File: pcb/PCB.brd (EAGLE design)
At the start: 42.5 x 42.5 mm, 18 parts

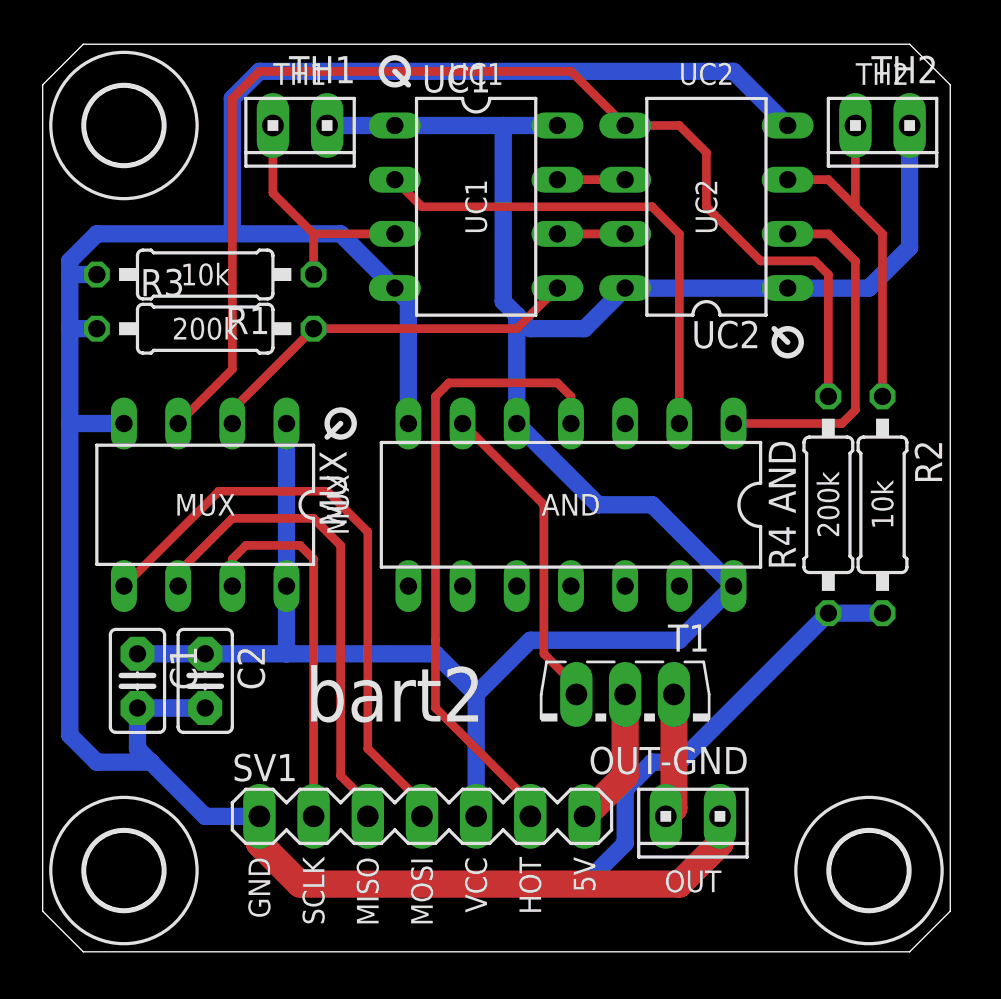
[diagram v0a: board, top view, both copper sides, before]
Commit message: Updated pcb
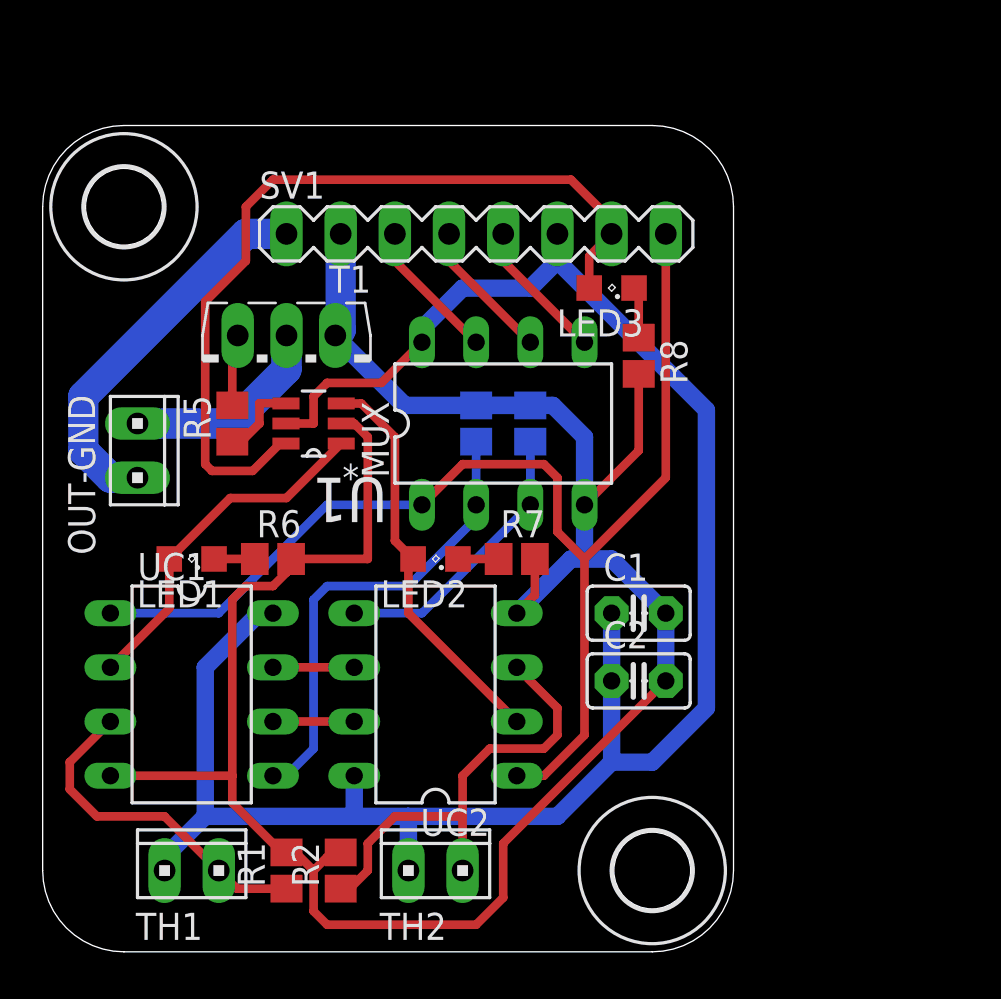
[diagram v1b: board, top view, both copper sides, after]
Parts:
- removed AND: 74HC21N, 74xx-eu:DIL14
- removed H2: MOUNT-HOLE3.6, holes:3,6
- added LED1, LED2, LED3: (no value), led:SML0805
- added R5: 1k, resistor:R0805
- added R6, R7, R8: 100, resistor:R0805
- added U1: SN74LVC1G11DBVR, parts:SOT95P280X145-6N
- R1, R2: device resistor:0207/10 -> resistor:R0805
- R3, R4: value 200k -> 100k; device resistor:0207/10 -> resistor:R0805
- SV1: device parts:MA07-1 -> parts:MA08-1
- moved TH2 40.7 mm to (18.4, 3.81), turned to 0 degrees
- moved TH1 35.3 mm to (6.99, 3.81), turned to 0 degrees
- moved OUT-GND 31.2 mm to (4.45, 23.5), turned to 270 degrees
- moved R2 30.6 mm to (14.0, 3.81), turned to 90 degrees
- moved R1 28.2 mm to (11.4, 3.81), turned to 90 degrees
- moved SV1 27.4 mm to (20.3, 33.7)
- moved UC1 26.5 mm to (6.99, 12.1)
- moved UC2 26.2 mm to (18.4, 12.1)
- moved C1 23.7 mm to (27.9, 15.9), turned to 0 degrees
- moved T1 23.1 mm to (11.4, 27.6)
- moved C2 20.3 mm to (27.9, 12.7), turned to 0 degrees
- moved MUX 14.5 mm to (21.6, 24.8), turned to 0 degrees
- moved R4 14.5 mm to (22.9, 24.8), flipped to the bottom, turned to 270 degrees
- moved R3 13.5 mm to (20.3, 24.8), flipped to the bottom, turned to 270 degrees
- moved H1 10.2 mm to (28.6, 3.81)
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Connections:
- new net N$2: LED3.C, R8.1
- new net N$3: R5.1, U1.4
- new net N$5: LED2.C, R7.1
- new net N$6: LED1.C, R6.1
- new net NRST: MUX.1, SV1.8, UC1.1, UC2.1
- net 5V: now also OUT-GND.1, SV1.1; no longer SV1.7, T1.2
- net GND: now also R6.2, R7.2, R8.2, SV1.2, T1.1, U1.2; no longer AND.7, OUT-GND.2, SV1.1
- net HOT: now also LED3.A, SV1.7, U1.6; no longer AND.4, SV1.6
- net MISO: now also SV1.4; no longer SV1.3
- net MOSI: now also SV1.5; no longer SV1.4
- net N$1: now also OUT-GND.2, T1.2; no longer OUT-GND.1, T1.1
- net N$4: now also R5.2; no longer AND.6
- net OUT1: now also LED1.A, U1.1; no longer AND.2
- net OUT2: now also LED2.A, U1.3; no longer AND.1
- net SCLK: now also SV1.3; no longer SV1.2
- net VCC: now also SV1.6, U1.5; no longer AND.14, AND.5, MUX.1, SV1.5, UC1.1, UC2.1
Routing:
- net NRST: track 0.00 -> 57.5 mm
- net GND: track 164.9 -> 115.0 mm
- net DRAAD2: track 55.9 -> 13.3 mm
- net MOSI: track 28.4 -> 6.66 mm
- net VCC: track 111.7 -> 93.7 mm
- net MISO: track 23.1 -> 6.66 mm
- net 5V: track 6.50 -> 18.3 mm
- net N$4: track 14.9 -> 3.38 mm
- net SCLK: track 17.7 -> 6.66 mm
- net HOT: track 29.7 -> 39.4 mm
- net OUT1: track 23.3 -> 16.5 mm
- net THERM2: track 16.9 -> 22.1 mm
- net THERM1: track 11.6 -> 16.1 mm
- net DRAAD1: track 18.2 -> 22.2 mm
- net N$3: track 0.00 -> 3.82 mm
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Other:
- board size 42.5 x 42.5 mm -> 32.4 x 38.7 mm
- board text added: "100k"
- board text added: "1k"
- board text added: "Bart2"
- board text added: "github.com/bwesterb/bart2"
- board text added: "nRST"
- board text added: "rev B"
- board text added: "uC1"
- board text added: "uC2"
- board text removed: "200k"
- board text removed: "AND"
- board text removed: "UC1"
- board text removed: "UC2"
- board text removed: "bart2"
